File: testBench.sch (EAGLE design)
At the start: 31 parts, among them IC1 NCS21911SN2T1G, IC2 NCS21911SN2T1G, IC3 NCS21911SN2T1G, IC4 NCS21911SN2T1G, IC5 NCS21911SN2T1G

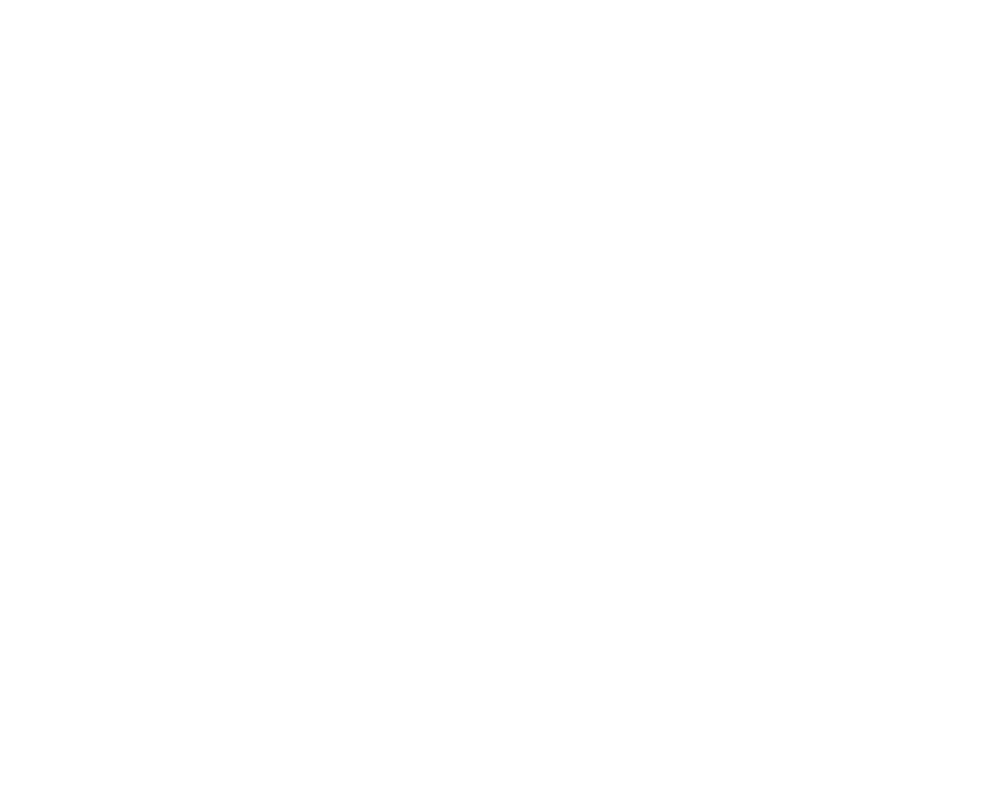
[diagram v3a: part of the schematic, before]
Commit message: PCB test bench version 8th
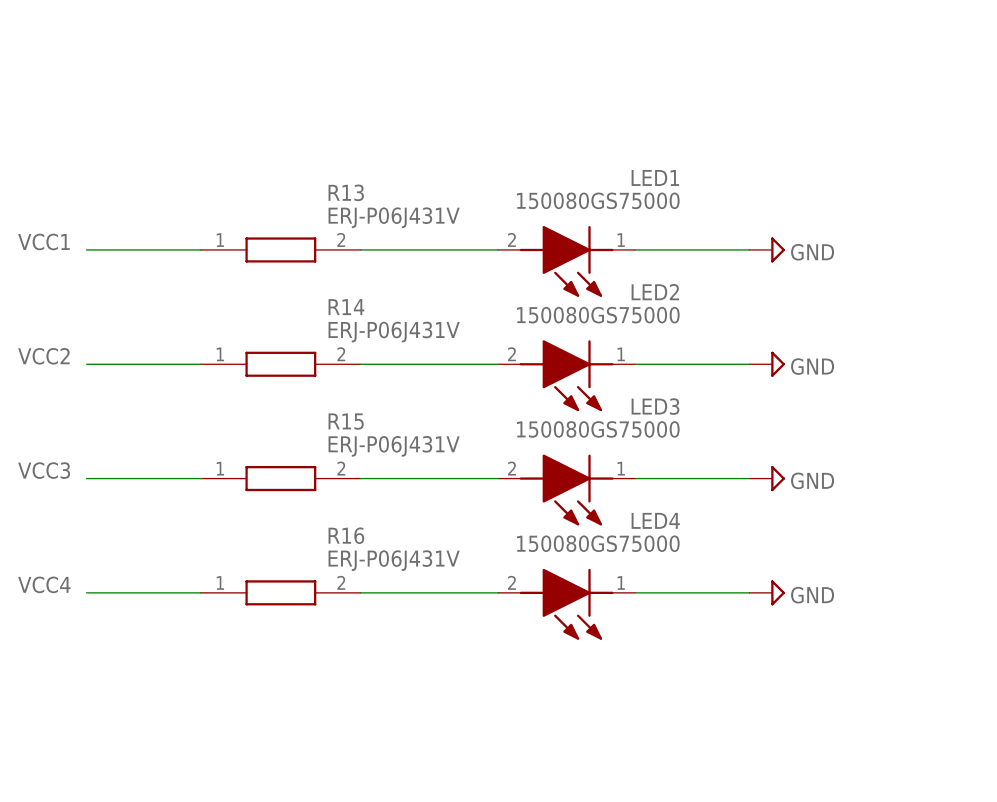
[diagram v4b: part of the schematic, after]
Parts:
- added LED1, LED2, LED3, LED4: 150080GS75000, SamacSys_Parts:150080GS75000
- added R13, R14, R15, R16: ERJ-P06J431V, SamacSys_Parts:ERJ-P06J431V
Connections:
- new net N$23: LED1.A, R13.2
- new net N$30: LED2.A, R14.2
- new net N$31: LED3.A, R15.2
- new net N$32: LED4.A, R16.2
- net GND: now also LED1.K, LED2.K, LED3.K, LED4.K
- net VCC1: now also R13.1
- net VCC2: now also R14.1
- net VCC3: now also R15.1
- net VCC4: now also R16.1
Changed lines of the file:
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@@
 <part name="TP7" library="SamacSys_Parts" deviceset="S1751-46R" device=""/>
 <part name="TP8" library="SamacSys_Parts" deviceset="S1751-46R" device=""/>
+<part name="LED1" library="SamacSys_Parts" deviceset="150080GS75000" device=""/>
+<part name="R13" library="SamacSys_Parts" deviceset="ERJ-P06J431V" device=""/>
+<part name="SUPPLY15" library="supply2" library_urn="urn:adsk.eagle:library:372" deviceset="GND" device=""/>
+<part name="LED2" library="SamacSys_Parts" deviceset="150080GS75000" device=""/>
+<part name="R14" library="SamacSys_Parts" deviceset="ERJ-P06J431V" device=""/>
+<part name="SUPPLY16" library="supply2" library_urn="urn:adsk.eagle:library:372" deviceset="GND" device=""/>
+<part name="LED3" library="SamacSys_Parts" deviceset="150080GS75000" device=""/>
+<part name="R15" library="SamacSys_Parts" deviceset="ERJ-P06J431V" device=""/>
+<part name="SUPPLY17" library="supply2" library_urn="urn:adsk.eagle:library:372" deviceset="GND" device=""/>
+<part name="LED4" library="SamacSys_Parts" deviceset="150080GS75000" device=""/>
+<part name="R16" library="SamacSys_Parts" deviceset="ERJ-P06J431V" device=""/>
+<part name="SUPPLY18" library="supply2" library_urn="urn:adsk.eagle:library:372" deviceset="GND" device=""/>
 </parts>
 <sheets>
@@
 <attribute name="NAME" x="53.34" y="-256.54" size="1.27" layer="95" rot="R270"/>
 </instance>
+<instance part="LED1" gate="G$1" x="-172.72" y="22.86" smashed="yes" rot="R180">
+<attribute name="NAME" x="-167.64" y="31.75" size="1.778" layer="95" rot="R180"/>
+<attribute name="VALUE" x="-167.64" y="29.21" size="1.778" layer="96" rot="R180"/>
+</instance>
+<instance part="R13" gate="G$1" x="-220.98" y="22.86" smashed="yes">
+<attribute name="NAME" x="-207.01" y="29.21" size="1.778" layer="95" align="center-left"/>
+<attribute name="VALUE" x="-207.01" y="26.67" size="1.778" layer="96" align="center-left"/>
+</instance>
+<instance part="SUPPLY15" gate="GND" x="-157.48" y="22.86" smashed="yes" rot="R90">
+<attribute name="VALUE" x="-150.495" y="23.495" size="1.778" layer="96" rot="R180"/>
+</instance>
+<instance part="LED2" gate="G$1" x="-172.72" y="10.16" smashed="yes" rot="R180">
+<attribute name="NAME" x="-167.64" y="19.05" size="1.778" layer="95" rot="R180"/>
+<attribute name="VALUE" x="-167.64" y="16.51" size="1.778" layer="96" rot="R180"/>
+</instance>
+<instance part="R14" gate="G$1" x="-220.98" y="10.16" smashed="yes">
+<attribute name="NAME" x="-207.01" y="16.51" size="1.778" layer="95" align="center-left"/>
+<attribute name="VALUE" x="-207.01" y="13.97" size="1.778" layer="96" align="center-left"/>
+</instance>
+<instance part="SUPPLY16" gate="GND" x="-157.48" y="10.16" smashed="yes" rot="R90">
+<attribute name="VALUE" x="-150.495" y="10.795" size="1.778" layer="96" rot="R180"/>
+</instance>
+<instance part="LED3" gate="G$1" x="-172.72" y="-2.54" smashed="yes" rot="R180">
+<attribute name="NAME" x="-167.64" y="6.35" size="1.778" layer="95" rot="R180"/>
+<attribute name="VALUE" x="-167.64" y="3.81" size="1.778" layer="96" rot="R180"/>
+</instance>
+<instance part="R15" gate="G$1" x="-220.98" y="-2.54" smashed="yes">
+<attribute name="NAME" x="-207.01" y="3.81" size="1.778" layer="95" align="center-left"/>
+<attribute name="VALUE" x="-207.01" y="1.27" size="1.778" layer="96" align="center-left"/>
+</instance>
+<instance part="SUPPLY17" gate="GND" x="-157.48" y="-2.54" smashed="yes" rot="R90">
+<attribute name="VALUE" x="-150.495" y="-1.905" size="1.778" layer="96" rot="R180"/>
+</instance>
+<instance part="LED4" gate="G$1" x="-172.72" y="-15.24" smashed="yes" rot="R180">
+<attribute name="NAME" x="-167.64" y="-6.35" size="1.778" layer="95" rot="R180"/>
+<attribute name="VALUE" x="-167.64" y="-8.89" size="1.778" layer="96" rot="R180"/>
+</instance>
+<instance part="R16" gate="G$1" x="-220.98" y="-15.24" smashed="yes">
+<attribute name="NAME" x="-207.01" y="-8.89" size="1.778" layer="95" align="center-left"/>
+<attribute name="VALUE" x="-207.01" y="-11.43" size="1.778" layer="96" align="center-left"/>
+</instance>
+<instance part="SUPPLY18" gate="GND" x="-157.48" y="-15.24" smashed="yes" rot="R90">
+<attribute name="VALUE" x="-150.495" y="-14.605" size="1.778" layer="96" rot="R180"/>
+</instance>
 </instances>
 <busses>
@@
 <wire x1="68.58" y1="-243.84" x2="76.2" y2="-243.84" width="0.1524" layer="91"/>
 <label x="78.74" y="-243.84" size="1.778" layer="95"/>
+</segment>
+<segment>
+<pinref part="LED1" gate="G$1" pin="K"/>
+<wire x1="-172.72" y1="22.86" x2="-160.02" y2="22.86" width="0.1524" layer="91"/>
+<pinref part="SUPPLY15" gate="GND" pin="GND"/>
+</segment>
+<segment>
+<pinref part="LED2" gate="G$1" pin="K"/>
+<wire x1="-172.72" y1="10.16" x2="-160.02" y2="10.16" width="0.1524" layer="91"/>
+<pinref part="SUPPLY16" gate="GND" pin="GND"/>
+</segment>
+<segment>
+<pinref part="LED3" gate="G$1" pin="K"/>
+<wire x1="-172.72" y1="-2.54" x2="-160.02" y2="-2.54" width="0.1524" layer="91"/>
+<pinref part="SUPPLY17" gate="GND" pin="GND"/>
+</segment>
+<segment>
+<pinref part="LED4" gate="G$1" pin="K"/>
+<wire x1="-172.72" y1="-15.24" x2="-160.02" y2="-15.24" width="0.1524" layer="91"/>
+<pinref part="SUPPLY18" gate="GND" pin="GND"/>
 </segment>
 </net>
@@
 <label x="25.4" y="-233.68" size="1.778" layer="95"/>
 </segment>
+<segment>
+<pinref part="R16" gate="G$1" pin="1"/>
+<wire x1="-220.98" y1="-15.24" x2="-233.68" y2="-15.24" width="0.1524" layer="91"/>
+<label x="-241.3" y="-15.24" size="1.778" layer="95"/>
+</segment>
 </net>
 <net name="VCC3" class="0">
@@
 <label x="10.16" y="-124.46" size="1.778" layer="95"/>
 </segment>
+<segment>
+<pinref part="R15" gate="G$1" pin="1"/>
+<wire x1="-220.98" y1="-2.54" x2="-233.68" y2="-2.54" width="0.1524" layer="91"/>
+<label x="-241.3" y="-2.54" size="1.778" layer="95"/>
+</segment>
 </net>
 <net name="VCC2" class="0">
@@
 <label x="22.86" y="-30.48" size="1.778" layer="95"/>
 </segment>
+<segment>
+<pinref part="R14" gate="G$1" pin="1"/>
+<wire x1="-220.98" y1="10.16" x2="-233.68" y2="10.16" width="0.1524" layer="91"/>
+<label x="-241.3" y="10.16" size="1.778" layer="95"/>
+</segment>
 </net>
 <net name="VCC1" class="0">
@@
 <label x="15.24" y="35.56" size="1.778" layer="95"/>
 </segment>
+<segment>
+<pinref part="R13" gate="G$1" pin="1"/>
+<wire x1="-220.98" y1="22.86" x2="-233.68" y2="22.86" width="0.1524" layer="91"/>
+<label x="-241.3" y="22.86" size="1.778" layer="95"/>
+</segment>
 </net>
 <net name="EMPTY" class="0">
@@
 </segment>
 </net>
+<net name="N$23" class="0">
+<segment>
+<pinref part="R13" gate="G$1" pin="2"/>
+<pinref part="LED1" gate="G$1" pin="A"/>
+<wire x1="-203.2" y1="22.86" x2="-187.96" y2="22.86" width="0.1524" layer="91"/>
+</segment>
+</net>
+<net name="N$30" class="0">
+<segment>
+<pinref part="R14" gate="G$1" pin="2"/>
+<pinref part="LED2" gate="G$1" pin="A"/>
+<wire x1="-203.2" y1="10.16" x2="-187.96" y2="10.16" width="0.1524" layer="91"/>
+</segment>
+</net>
+<net name="N$31" class="0">
+<segment>
+<pinref part="R15" gate="G$1" pin="2"/>
+<pinref part="LED3" gate="G$1" pin="A"/>
+<wire x1="-203.2" y1="-2.54" x2="-187.96" y2="-2.54" width="0.1524" layer="91"/>
+</segment>
+</net>
+<net name="N$32" class="0">
+<segment>
+<pinref part="R16" gate="G$1" pin="2"/>
+<pinref part="LED4" gate="G$1" pin="A"/>
+<wire x1="-203.2" y1="-15.24" x2="-187.96" y2="-15.24" width="0.1524" layer="91"/>
+</segment>
+</net>
